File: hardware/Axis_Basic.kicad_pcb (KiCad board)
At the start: 4 copper layers, 42 x 42 mm, 58 parts, among them J1 USB_C_Receptacle_USB2.0, J2 JST_PH, J3 JST_SH, J4 JST_PH, J5 2.56mm Dupont Connector, J6 Screw_Terminal_01x04, J7 Conn_ARM_JTAG_SWD_10, J8 Conn_01x07_Pin, SW1 RKB2SJK, SW2 RKB2SJK, U1 UA78M33CDCYR, U3 TMC2209-LA, U4 AT25040B-MAHL-T, Y1 ECS-.327-12.5-34B-TR

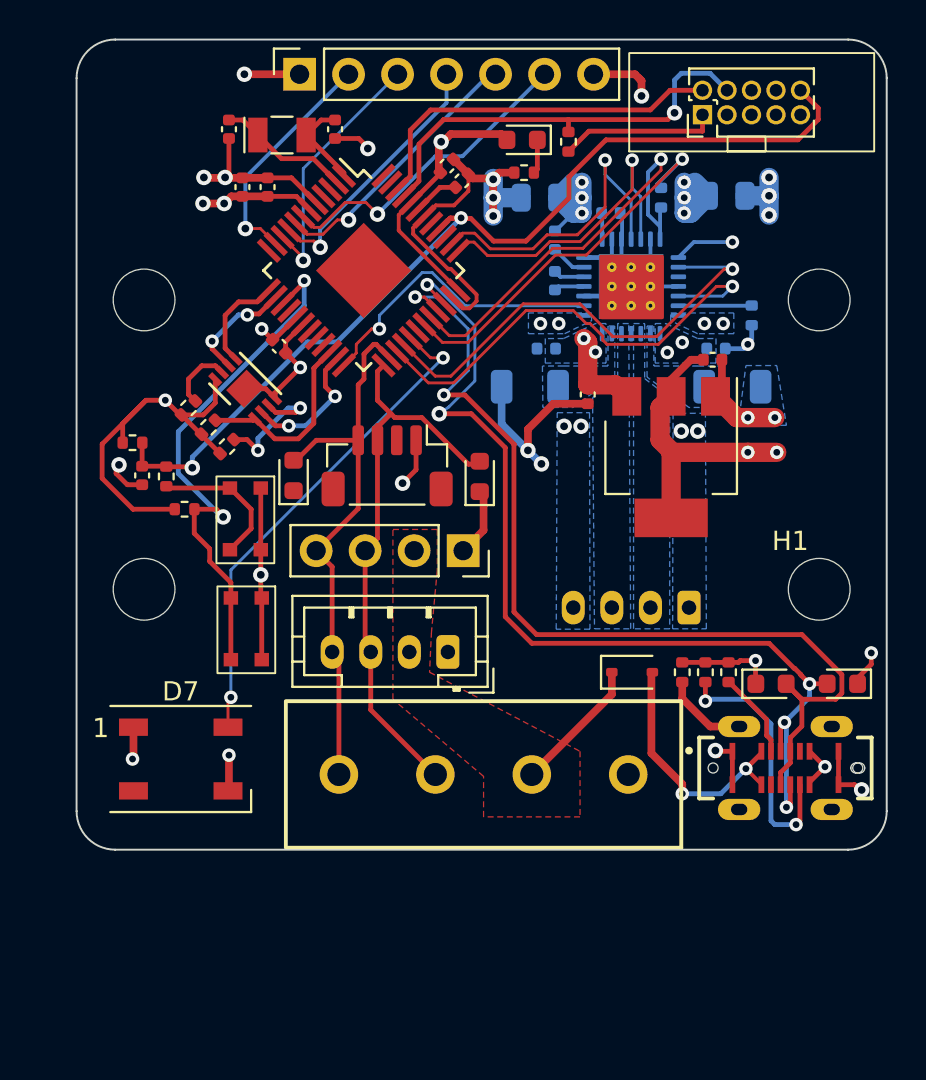
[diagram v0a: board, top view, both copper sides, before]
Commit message: PCB layout and routing complete
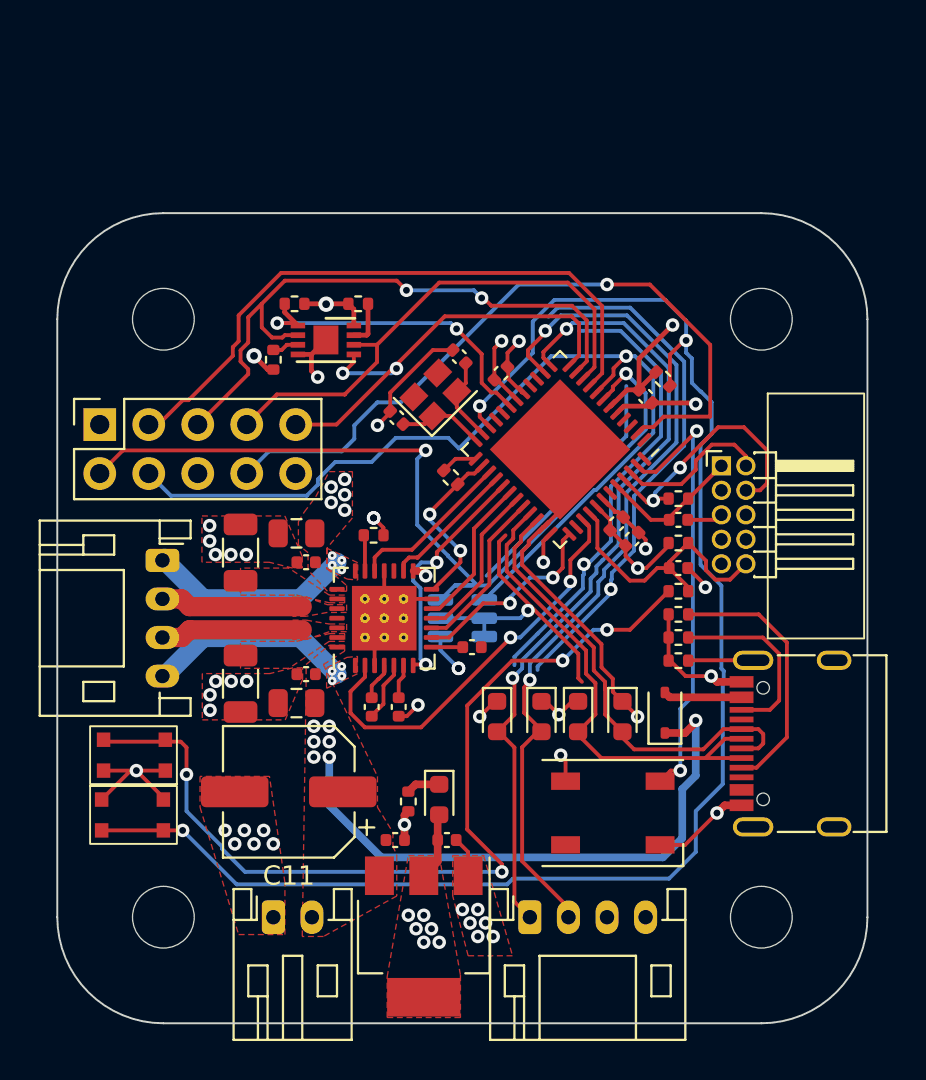
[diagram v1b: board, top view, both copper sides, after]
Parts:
- removed J7: Conn_ARM_JTAG_SWD_10, Connector_PinHeader_1.27mm:PinHeader_2x05_P1.27mm_Vertical
- removed J8: Conn_01x07_Pin, Connector_PinSocket_2.54mm:PinSocket_1x07_P2.54mm_Vertical
- added C18: 1pF, Capacitor_SMD:C_0402_1005Metric, F.Cu at (146.6, 89.6)
- added U5: AT25040B-MAHL-T, Package_DFN_QFN:DFN-8-1EP_3x2mm_P0.5mm_EP1.3x1.5mm, F.Cu at (142.9, 85.6)
- C1: value 100n -> 0.47u Tant.
- C10: value 100n -> 22u; footprint Capacitor_SMD:C_0402_1005Metric -> Capacitor_SMD:C_0805_2012Metric
- C11: value 22n -> 47u; footprint Capacitor_SMD:C_0402_1005Metric -> Capacitor_SMD:CP_Elec_6.3x5.4; moved to F.Cu
- C12: value 2.2u -> 100n; moved to F.Cu
- C13, C14, C15, R14, R15, R7, R8: moved to F.Cu
- C16: value 22u -> 4.7u; footprint Capacitor_SMD:C_0805_2012Metric -> Capacitor_SMD:C_0402_1005Metric; moved to F.Cu
- C17: value 22u -> 1pF; footprint Capacitor_SMD:C_0805_2012Metric -> Capacitor_SMD:C_0402_1005Metric; moved to F.Cu
- C2: value 10u -> 22u Tant.
- C4: value 0.47u Tant. -> 22n
- C5: value 100n -> 2.2u
- C6: value 1u -> 100n
- C7: value 22u Tant. -> 100n
- C8: value 20p -> 100n
- C9: value 20p -> 22u; footprint Capacitor_SMD:C_0402_1005Metric -> Capacitor_SMD:C_0805_2012Metric
- D5: value GSEN3U003 -> XZMDK54W-1; footprint Diode_SMD:D_0603_1608Metric -> LED_SMD:LED_0603_1608Metric
- D6: value XZMDK54W-1 -> GSEN3U003; footprint LED_SMD:LED_0603_1608Metric -> Diode_SMD:D_0603_1608Metric
- J1: footprint GCT_USB4120-03-C_REVA:GCT_USB4120-03-C_REVA -> Connector_USB:USB_C_Receptacle_G-Switch_GT-USB-7010ASV
- J2: footprint Connector_JST:JST_PH_B4B-PH-K_1x04_P2.00mm_Vertical -> Connector_JST:JST_PH_S4B-PH-K_1x04_P2.00mm_Horizontal; moved to F.Cu
- J3: value JST_SH -> JST_PH; footprint Connector_JST:JST_SH_BM04B-SRSS-TB_1x04-1MP_P1.00mm_Vertical -> Connector_JST:JST_PH_S4B-PH-K_1x04_P2.00mm_Horizontal
- J4: value JST_PH -> S2B-PH-K-S; footprint Connector_JST:JST_PH_B4B-PH-K_1x04_P2.00mm_Vertical -> Connector_JST:JST_PH_S2B-PH-K_1x02_P2.00mm_Horizontal
- J5: value 2.56mm Dupont Connector -> 1175-1628-ND; footprint Connector_PinSocket_2.54mm:PinSocket_1x04_P2.54mm_Vertical -> Connector_PinHeader_1.27mm:PinHeader_2x05_P1.27mm_Horizontal
- J6: value Screw_Terminal_01x04 -> Conn_01x10; footprint Screw_Terminal:EBBA-04-C-SS-BU -> Connector_PinSocket_2.54mm:PinSocket_2x05_P2.54mm_Vertical
- U1: value UA78M33CDCYR -> TLV493D; footprint Package_TO_SOT_SMD:SOT-223-3_TabPin2 -> Package_TO_SOT_SMD:SOT-23-6; moved to B.Cu
- U2: value ~ -> UA78M33CDCYR; footprint Package_QFP:TQFP-48-1EP_7x7mm_P0.5mm_EP3.5x3.5mm -> Package_TO_SOT_SMD:SOT-223-3_TabPin2
- U3: value TMC2209-LA -> ATSAMD51G18A-MU; footprint Package_DFN_QFN:QFN-28-1EP_5x5mm_P0.5mm_EP3.35x3.35mm_ThermalVias -> Package_DFN_QFN:VQFN-48-1EP_7x7mm_P0.5mm_EP5.15x5.15mm; moved to F.Cu
- U4: value AT25040B-MAHL-T -> TMC2209-LA; footprint Package_DFN_QFN:DFN-8-1EP_3x2mm_P0.5mm_EP1.3x1.5mm -> Package_DFN_QFN:QFN-28-1EP_5x5mm_P0.5mm_EP3.35x3.35mm_ThermalVias
- Y1: value ECS-.327-12.5-34B-TR -> SG-210STF 48.0000ML0; footprint Crystal:Crystal_SMD_G8-2Pin_3.2x1.5mm -> Crystal:Crystal_SMD_2520-4Pin_2.5x2.0mm
- moved H2 46.7 mm to (134.5, 115.5)
- moved C2 35.5 mm to (149.2, 111.5), turned to 0 degrees
- moved H4 34.9 mm to (165.5, 84.5)
- moved U2 34.7 mm to (148.0, 116.5), turned to -90 degrees
- moved R10 33.1 mm to (147.2, 109.5), turned to -90 degrees
- moved D6 30.0 mm to (156.0, 105.1), turned to -90 degrees
- moved C11 29.9 mm to (141.0, 109.0), turned to 180 degrees
- moved C3 29.0 mm to (161.2, 97.4), turned to 0 degrees
- moved R6 28.8 mm to (161.2, 96.1)
- moved C8 28.3 mm to (141.9, 102.9), turned to 180 degrees
- moved C6 27.5 mm to (146.7, 104.6), turned to 90 degrees
- moved J2 27.4 mm to (134.4, 100.0), turned to -90 degrees
- moved R5 27.2 mm to (161.2, 98.6), turned to 0 degrees
- moved J6 26.9 mm to (131.2, 90.0), turned to 90 degrees
- moved R15 26.9 mm to (138.5, 96.6), turned to 90 degrees
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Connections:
- C1 pad 1: +3.3V -> VCC
- C10 pad 1: RESET -> VCC
- C11 pad 1: Net-(U3-CPI) -> VCC
- C11 pad 2: Net-(U3-CPO) -> GND
- C12 pad 1: Net-(U3-5VOUT) -> +3.3V
- C13 pad 1: VCC -> +3.3V
- C13 pad 2: Net-(U3-VCP) -> GND
- C14 pad 1: VCC -> +3.3V
- C15 pad 1: VCC -> +3.3V
- C16 pad 1: VCC -> +3.3V
- C17 pad 1: VCC -> GND
- C17 pad 2: GND -> Net-(U3-PA14/SERCOM2_2/SERCOM4_2)
- C3 pad 1: +3.3V -> RESET
- C4 pad 1: VCC -> Net-(U4-CPI)
- C4 pad 2: GND -> Net-(U4-CPO)
- C5 pad 1: +3.3V -> Net-(U4-5VOUT)
- C6 pad 1: Net-(U2-VDDCORE) -> VCC
- C6 pad 2: GND -> Net-(U4-VCP)
- C7 pad 1: +3.3V -> VCC
- C8 pad 1: GND -> VCC
- C8 pad 2: Net-(U2-PA00/EINT0/SERCOM1.0) -> GND
- C9 pad 1: GND -> VCC
- C9 pad 2: Net-(U2-PA01/EINT1/SERCOM1.1) -> GND
- D2 pad 2: SCL -> SCL2
- D3 pad 2: SDA -> SDA2
- D5 pad 1: GND -> Net-(D5-K)
- D5 pad 2: D- -> +3.3V
- D6 pad 1: Net-(D6-K) -> GND
- D6 pad 2: +3.3V -> D-
- J3 pad 1: GND -> SCL2
- J3 pad 2: unconnected-(J3-Pad2) -> SDA2
- J3 pad 3: SDA -> unconnected-(J3-Pad3)
- J3 pad 4: SCL -> GND
- J5 pad 1: GND -> +3.3V
- J5 pad 2: VCC -> SWDIO
- J5 pad 3: SDA -> GND
- J5 pad 4: SCL -> SWCLK
- J6 pad 2: VCC -> SDA1
- J6 pad 3: SDA -> ETH_CS
- J6 pad 4: SCL -> SCL1
- R10 pad 1: Net-(D6-K) -> Net-(D5-K)
- R11 pad 2: Net-(U4-~{WP}) -> Net-(U5-~{WP})
- R12 pad 2: Net-(U4-~{HOLD}) -> Net-(U5-~{HOLD})
- R8 pad 1: Net-(U3-STDBY) -> Net-(U4-STDBY)
- U1 pad 1: GND -> SCL1
- U1 pad 2: +3.3V -> GND
- U1 pad 3: VCC -> GND
- U2 pad 1: Net-(U2-PA00/EINT0/SERCOM1.0) -> GND
- U2 pad 2: Net-(U2-PA01/EINT1/SERCOM1.1) -> +3.3V
- U2 pad 3: unconnected-(U2-PA02/EINT2/AIN0/Y0/VOUT-Pad3) -> VCC
- U3 pad 1: MOTOR_B2 -> unconnected-(U3-PA00/SERCOM1_0-Pad1)
- U3 pad 10: GND -> SCK
- U3 pad 11: DIAG -> MISO
- U3 pad 12: INDEX -> MOSI
- U3 pad 13: GND -> SCL2
- U3 pad 14: UART_RX -> SDA2
- U3 pad 15: +3.3V -> unconnected-(U3-PA10/SERCOM0_2/SERCOM2_2-Pad15)
- U3 pad 16: STEP -> unconnected-(U3-PA11/SERCOM0_3/SERCOM2_3-Pad16)
- U3 pad 17: unconnected-(U3-VREF-Pad17) -> +3.3V
- U3 pad 19: DIR -> EEPROM_CS
- U3 pad 2: EN -> Net-(J6-Pin_8)
- U3 pad 20: Net-(U3-STDBY) -> unconnected-(U3-PB11/SERCOM4_3-Pad20)
- U3 pad 21: MOTOR_A1 -> unconnected-(U3-PA12/SERCOM2_0/SERCOM4_1-Pad21)
- U3 pad 22: VCC -> User_Input
- U3 pad 23: /BRA -> Net-(U3-PA14/SERCOM2_2/SERCOM4_2)
- U3 pad 24: MOTOR_B1 -> Net-(U3-PA15/SERCOM2_3/SERCOM4_3)
- U3 pad 25: unconnected-(U3-NC-Pad25) -> UART_TX
- U3 pad 26: MOTOR_A2 -> UART_RX
- U3 pad 27: /BRB -> DIR
- U3 pad 28: VCC -> STEP
- U3 pad 29: GND -> Spread
- U3 pad 3: GND -> unconnected-(U3-PA02-Pad3)
- U3 pad 4: Net-(U3-CPO) -> unconnected-(U3-PA03-Pad4)
- U3 pad 5: Net-(U3-CPI) -> GND
- U3 pad 6: Net-(U3-VCP) -> +3.3V
- U3 pad 7: GND -> SDA1
- U3 pad 8: Net-(U3-5VOUT) -> SCL1
- U3 pad 9: GND -> ETH_CS
- U4 pad 1: EEPROM_CS -> MOTOR_B2
- U4 pad 2: EEPROM_MISO -> EN
- U4 pad 3: Net-(U4-~{WP}) -> GND
- U4 pad 4: GND -> Net-(U4-CPO)
- U4 pad 5: EEPROM_MOSI -> Net-(U4-CPI)
- U4 pad 6: EEPROM_SCK -> Net-(U4-VCP)
- U4 pad 7: Net-(U4-~{HOLD}) -> Spread
- U4 pad 8: +3.3V -> Net-(U4-5VOUT)
- U4 pad 9: GND -> MOT_M0
- Y1 pad 1: Net-(U2-PA01/EINT1/SERCOM1.1) -> Net-(U3-PA15/SERCOM2_3/SERCOM4_3)
- Y1 pad 2: Net-(U2-PA00/EINT0/SERCOM1.0) -> Net-(U3-PA14/SERCOM2_2/SERCOM4_2)
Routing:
- net User_Input: track 27.9 -> 80.8 mm, vias 2 -> 3
- net SCL1: track 0.00 -> 48.5 mm, vias 0 -> 1
- net SDA1: track 0.00 -> 46.5 mm, vias 0 -> 2
- net SDA2: track 0.00 -> 45.3 mm, vias 0 -> 2
- net GND: track 109.5 -> 154.7 mm, vias 24 -> 40
- net SCL2: track 0.00 -> 42.0 mm, vias 0 -> 2
- net Net-(R5-Pad1): track 7.45 -> 48.4 mm, vias 0 -> 4
- net Net-(J6-Pin_8): track 0.00 -> 37.7 mm, vias 0 -> 1
- net RESET: track 50.5 -> 14.4 mm, vias 2 -> 0
- net +3.3V: track 73.7 -> 38.6 mm, vias 10 -> 16
- net ETH_CS: track 0.00 -> 32.9 mm
- net MISO: track 0.00 -> 32.7 mm, vias 0 -> 2
- net SDA: track 29.6 -> 0.00 mm
- net SCL: track 29.1 -> 0.00 mm
- net SCK: track 0.00 -> 27.7 mm
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- added copper zone on F.Cu, net +3.3V
- added copper zone on F.Cu, net /BRA
- added copper zone on F.Cu, net /BRB
- added copper zone on F.Cu, net GND
- added copper zone on F.Cu, net MOTOR_A1
- added copper zone on F.Cu, net MOTOR_A2
- added copper zone on F.Cu, net MOTOR_B1
- added copper zone on F.Cu, net MOTOR_B2
- removed copper zone on B.Cu, net /BRA
- removed copper zone on B.Cu, net /BRB
- removed copper zone on B.Cu, net GND
- removed copper zone on B.Cu, net MOTOR_A1
- removed copper zone on In2.Cu, net MOTOR_A1
- removed copper zone on B.Cu, net MOTOR_A2
- removed copper zone on B.Cu, net MOTOR_B1
- removed copper zone on B.Cu, net MOTOR_B2
- removed copper zone on In2.Cu, net MOTOR_B2
- removed copper zone on B.Cu, net VCC
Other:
- outline, holes or cut-outs redrawn
